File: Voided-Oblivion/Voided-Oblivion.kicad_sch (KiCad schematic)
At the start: 39 parts, among them J4 SM03B-SRSS-TB, SW1 boot, SW2 reset, U1 RP2350_80QFN, U3 W25Q128JVS, U4 W25Q128JVS, Y1 ABM8-272-T3

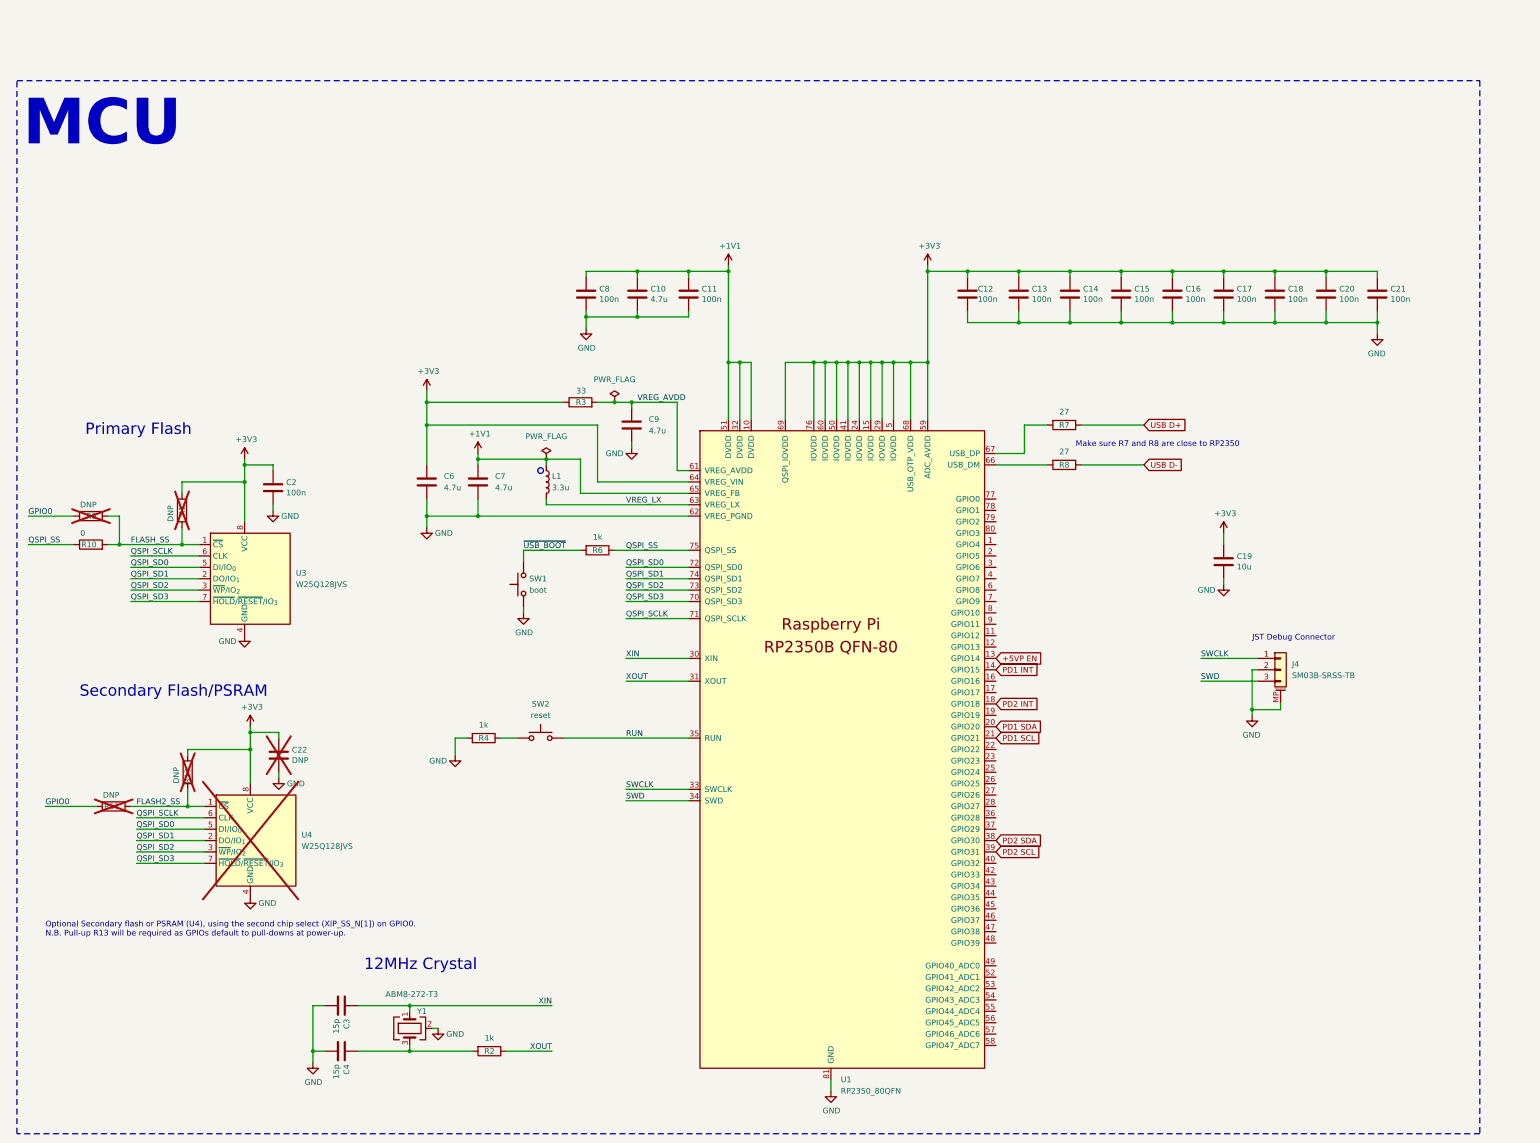
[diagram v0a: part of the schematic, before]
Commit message: update.com
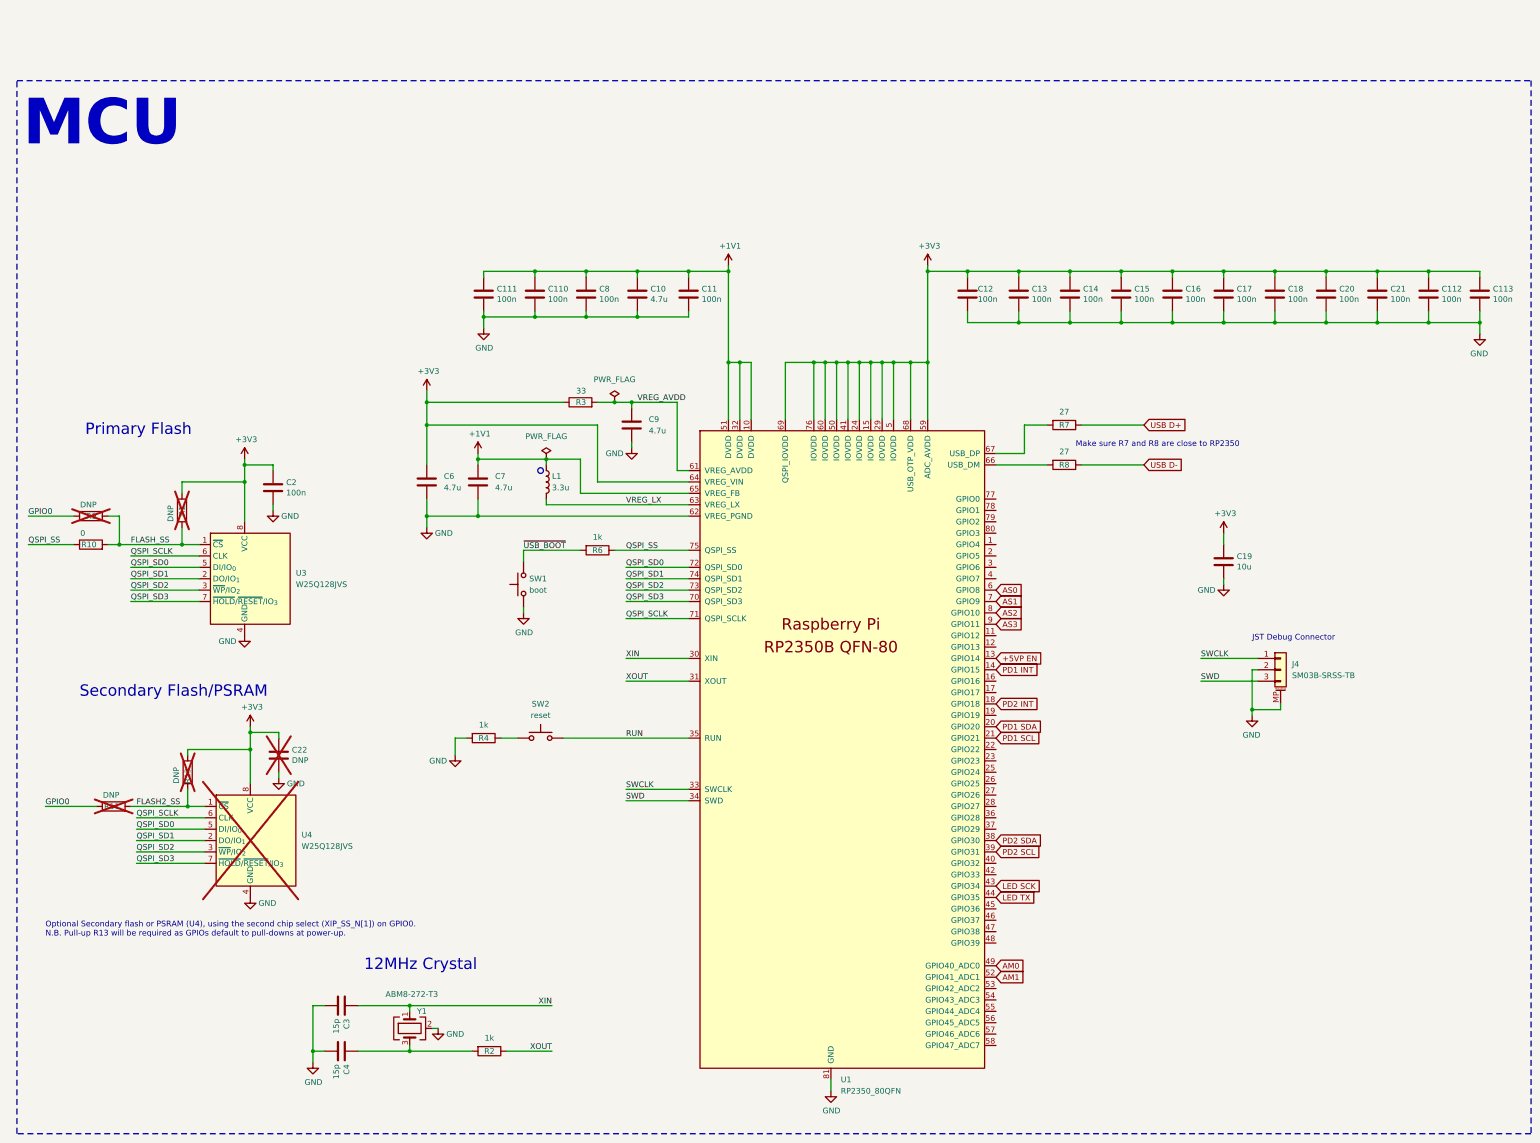
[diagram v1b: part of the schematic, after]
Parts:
- added C110, C111, C112, C113: 100n, Capacitor_SMD:C_0402_1005Metric, symbol Device:C
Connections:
- net +1V1: now also C110.1, C111.1
- net +3V3: now also C112.1, C113.1
- net GND: now also C110.2, C111.2, C112.2, C113.2
- net LED SCK: now reaches U1.43 (GPIO34)
- net LED TX: now reaches U1.44 (GPIO35)
- net AM0: now reaches U1.49 (GPIO40_ADC0)
- net AM1: now reaches U1.52 (GPIO41_ADC1)
- net AS0: now reaches U1.6 (GPIO8)
- net AS1: now reaches U1.7 (GPIO9)
- net AS2: now reaches U1.8 (GPIO10)
- net AS3: now reaches U1.9 (GPIO11)

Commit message: update
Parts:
- C10, C6, C7, C9: LCSC (none) -> C23733; MPN (none) -> CL05A475MP5NRNC; Manufacturer (none) -> Samsung Electro-Mechanics
- C11, C110, C111, C112, C113, C12, C13, C14, C15, C16, C17, C18, C2, C20, C21, C8: LCSC (none) -> C307331; MPN (none) -> CL05B104KB54PNC; Manufacturer (none) -> Samsung Electro-Mechanics
- C19: LCSC (none) -> C95841; MPN (none) -> CL21B106KOQNNNE; Manufacturer (none) -> Samsung Electro-Mechanics
- C22, R1, R11, R13, R9, U4: BOM Comments (none) -> DNP - do not populate; DNP (none) -> DNP
- C3, C4: LCSC (none) -> C1548; MPN (none) -> 0402CG150J500NT; Manufacturer (none) -> Guangdong Fenghua (FH)
- J4: LCSC (none) -> C160403; MPN (none) -> SM03B-SRSS-TB(LF)(SN); Manufacturer (none) -> JST
- L1: LCSC (none) -> C3221749; MPN (none) -> VLS201610CX-3R3M-1; Manufacturer (none) -> TDK
- R10: LCSC (none) -> C17168; MPN (none) -> 0402WGF0000TCE; Manufacturer (none) -> UNI-ROYAL
- R2, R4, R6: LCSC (none) -> C11702; MPN (none) -> 0402WGF1001TCE; Manufacturer (none) -> UNI-ROYAL
- R3: LCSC (none) -> C138002; MPN (none) -> RC0402FR-0733RL; Manufacturer (none) -> Yageo
- R7, R8: LCSC (none) -> C138021; MPN (none) -> RC0402FR-0727RL; Manufacturer (none) -> Yageo
- U1: LCSC (none) -> C42415655; MPN (none) -> RP2350B; Manufacturer (none) -> Raspberry Pi
- U3: LCSC (none) -> C97521; MPN (none) -> W25Q128JVSIQ; Manufacturer (none) -> Winbond
- Y1: LCSC (none) -> C20625731; MPN (none) -> ABM8-272-T3; Manufacturer (none) -> Abracon
